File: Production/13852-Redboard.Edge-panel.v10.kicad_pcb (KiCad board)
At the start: 2 copper layers, 101.6 x 38.1 mm, 72 parts, among them J1 CONN_025MM, J17 QWIIC_CONNECTORJS-1MM, J2 CONN_03X2SMT, J20 POWER_JACKSMD, J4 USB_MICRO-B, J5 CONN_04, J6 CONN_04, Q1 MOSFET-SI2309DS, Q2 BSS138, Q3 BSS138, U1 CH340GSMD, U2 MIC5205-3.3V, U3 Standoff_Grounding, U4 ATMEGA328, U5 Standoff_Grounding, U6 LM1117, Y1 RESONATOR-16MHZ, Y2 CRYSTAL-12MHZ

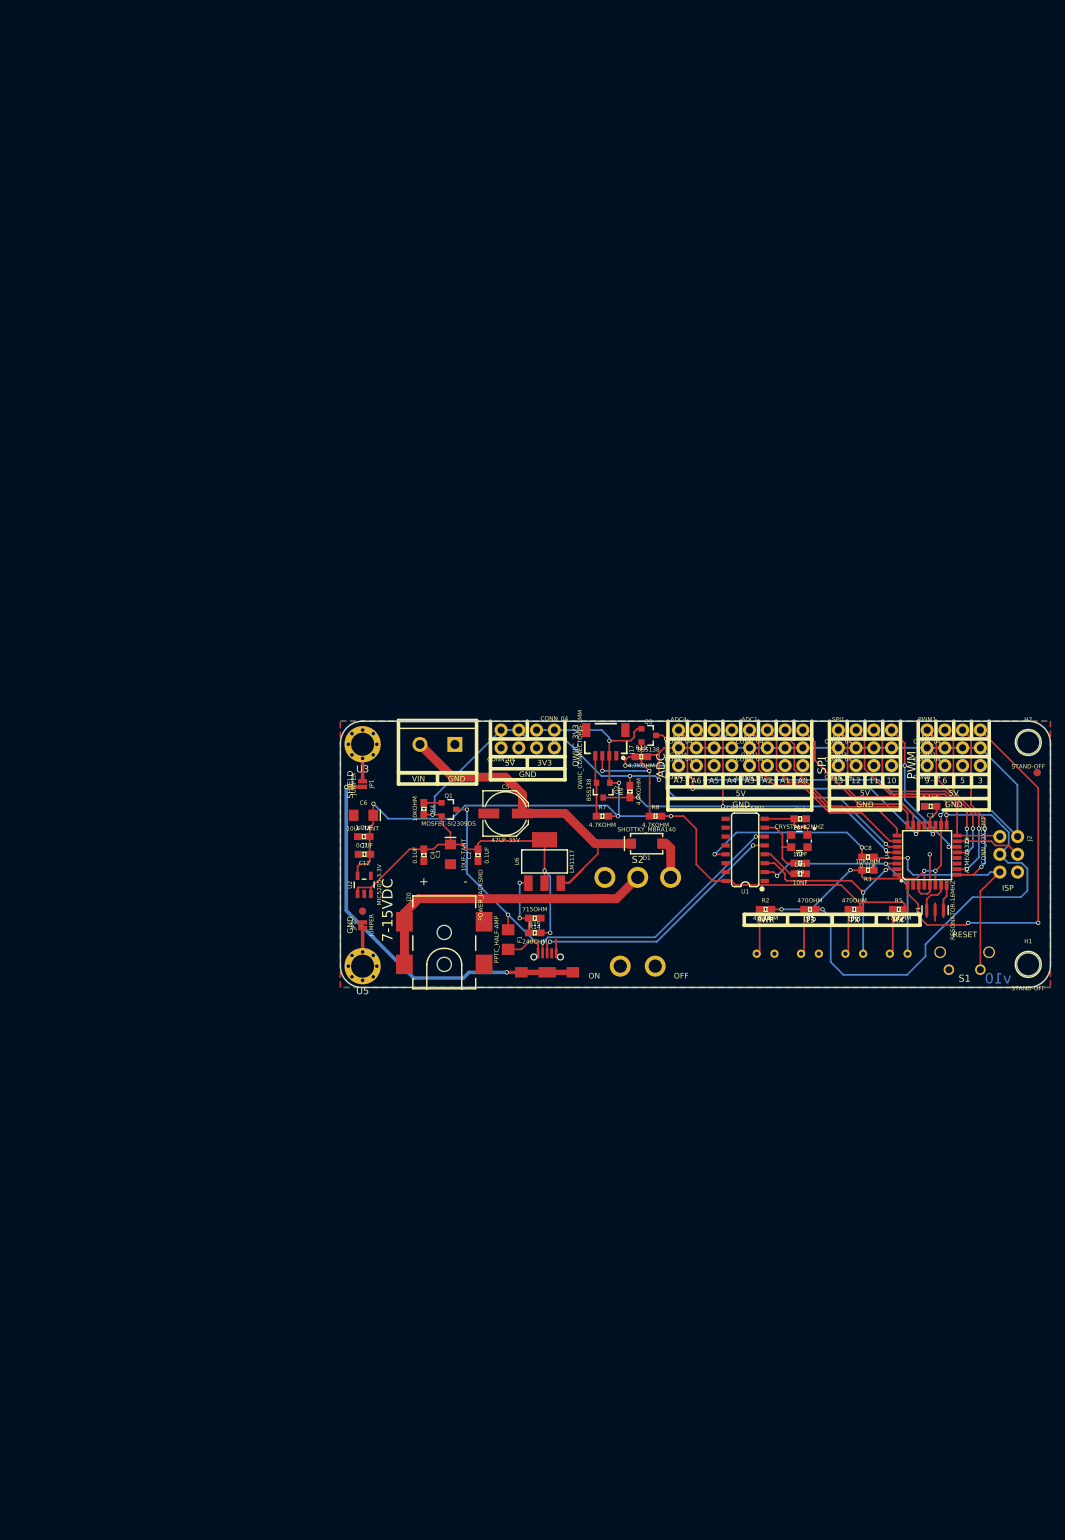
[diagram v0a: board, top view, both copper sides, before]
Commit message: panel
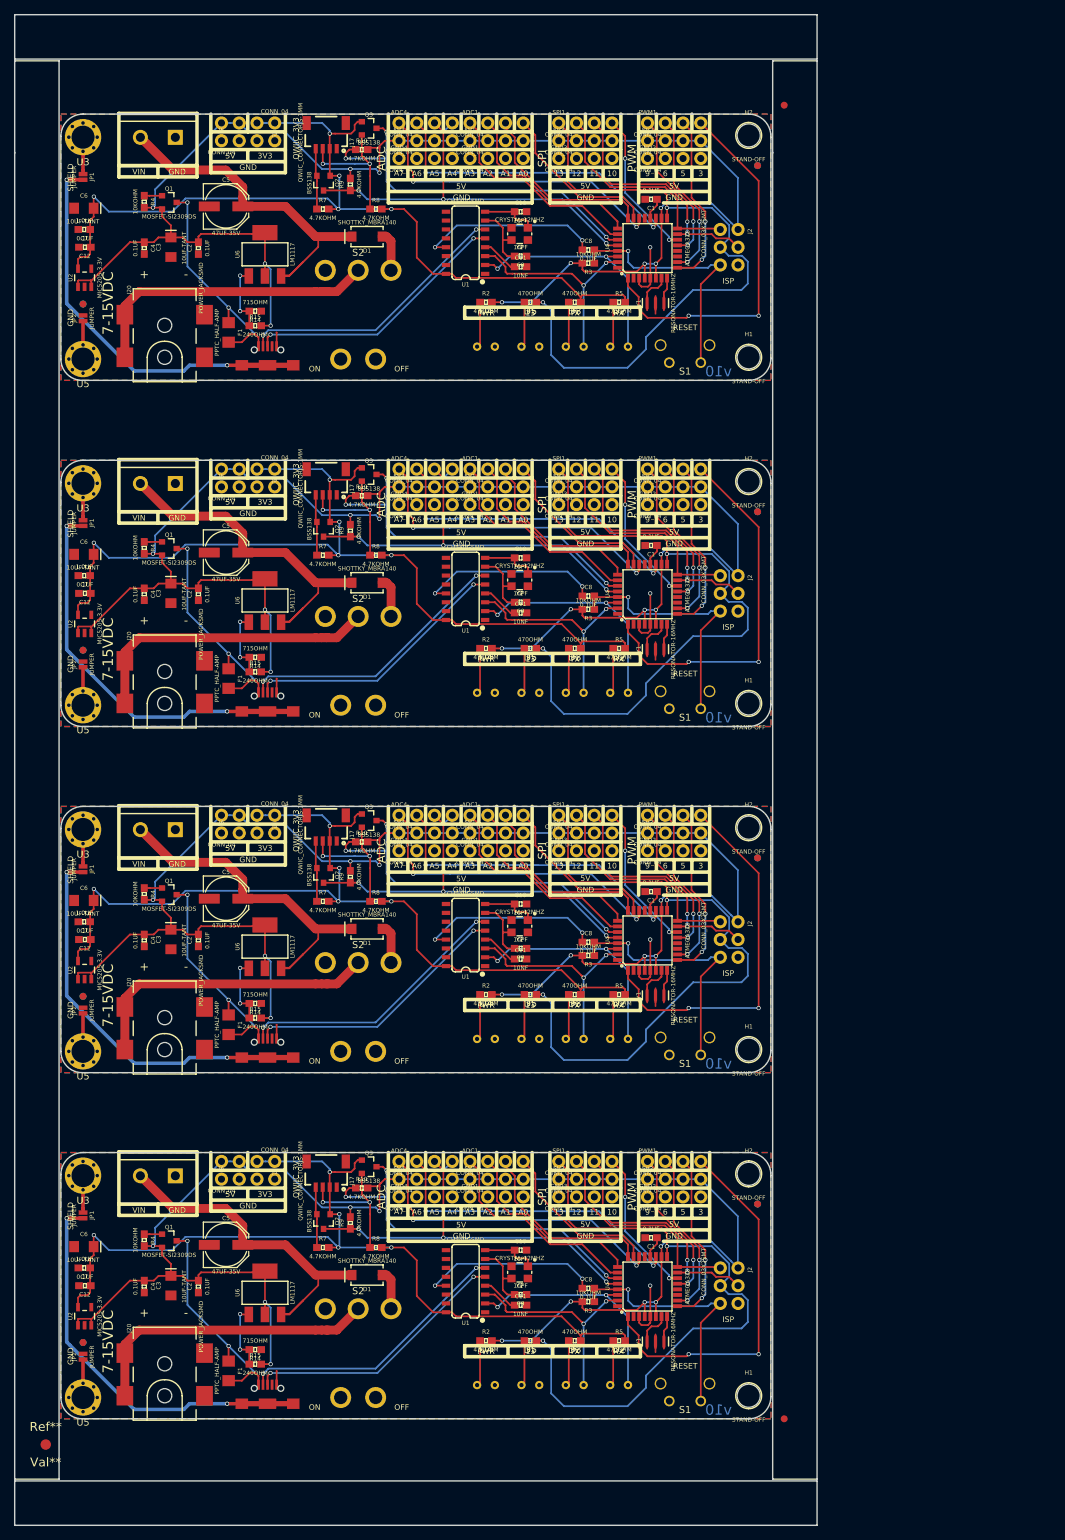
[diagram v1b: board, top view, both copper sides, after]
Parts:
- added 5V1: CONN_04, Connectors:1X04_NO_SILK, F.Cu at (119.5, -3.81)
- added 5V1: CONN_04, Connectors:1X04_NO_SILK, F.Cu at (119.5, 45.7)
- added 5V1: CONN_04, Connectors:1X04_NO_SILK, F.Cu at (119.5, 95.2)
- added 5V2: CONN_04, Connectors:1X04_NO_SILK, F.Cu at (144.9, -3.81)
- added 5V2: CONN_04, Connectors:1X04_NO_SILK, F.Cu at (144.9, 45.7)
- added 5V2: CONN_04, Connectors:1X04_NO_SILK, F.Cu at (144.9, 95.2)
- added 5V3: CONN_04, Connectors:1X04_NO_SILK, F.Cu at (132.2, -3.81)
- added 5V3: CONN_04, Connectors:1X04_NO_SILK, F.Cu at (132.2, 45.7)
- added 5V3: CONN_04, Connectors:1X04_NO_SILK, F.Cu at (132.2, 95.2)
- added 5V4: CONN_04, Connectors:1X04_NO_SILK, F.Cu at (109.3, -3.81)
- added 5V4: CONN_04, Connectors:1X04_NO_SILK, F.Cu at (109.3, 45.7)
- added 5V4: CONN_04, Connectors:1X04_NO_SILK, F.Cu at (109.3, 95.2)
- added ?: , Aesthetics:FIDUCIAL-1X2-no.paste, F.Cu at (164.5, 179.1)
- added ?: , Aesthetics:FIDUCIAL-1X2-no.paste, F.Cu at (164.5, -8.89)
- added ADC1: CONN_04, Connectors:1X04_NO_SILK, F.Cu at (119.5, -6.35)
- added ADC1: CONN_04, Connectors:1X04_NO_SILK, F.Cu at (119.5, 43.2)
- added ADC1: CONN_04, Connectors:1X04_NO_SILK, F.Cu at (119.5, 92.7)
- added ADC4: CONN_04, Connectors:1X04_NO_SILK, F.Cu at (109.3, -6.35)
- added ADC4: CONN_04, Connectors:1X04_NO_SILK, F.Cu at (109.3, 43.2)
- added ADC4: CONN_04, Connectors:1X04_NO_SILK, F.Cu at (109.3, 92.7)
- added C1: 0.1UF, Capacitors:0603, F.Cu at (145.4, 4.57)
- added C1: 0.1UF, Capacitors:0603, F.Cu at (145.4, 54.1)
- added C1: 0.1UF, Capacitors:0603, F.Cu at (145.4, 103.6)
- added C10: 10PF, Capacitors:0603, F.Cu at (126.7, 6.35)
- added C10: 10PF, Capacitors:0603, F.Cu at (126.7, 55.9)
- added C10: 10PF, Capacitors:0603, F.Cu at (126.7, 105.4)
- added C11: 10NF, Capacitors:0603, F.Cu at (126.7, 14.2)
- added C11: 10NF, Capacitors:0603, F.Cu at (126.7, 63.8)
- added C11: 10NF, Capacitors:0603, F.Cu at (126.7, 113.3)
- added C12: 0.1UF, Capacitors:0603, F.Cu at (64.4, 11.4)
- added C12: 0.1UF, Capacitors:0603, F.Cu at (64.4, 61.0)
- added C12: 0.1UF, Capacitors:0603, F.Cu at (64.4, 110.5)
- added C2: 0.1UF, Capacitors:0603, F.Cu at (80.6, 11.6)
- added C2: 0.1UF, Capacitors:0603, F.Cu at (80.6, 61.1)
- added C2: 0.1UF, Capacitors:0603, F.Cu at (80.6, 110.6)
- added C3: 10UF-TANT, Capacitors:EIA3216, F.Cu at (76.7, 11.4)
- added C3: 10UF-TANT, Capacitors:EIA3216, F.Cu at (76.7, 61.0)
- added C3: 10UF-TANT, Capacitors:EIA3216, F.Cu at (76.7, 110.5)
- added C4: 0.1UF, Capacitors:0603, F.Cu at (72.9, 11.6)
- added C4: 0.1UF, Capacitors:0603, F.Cu at (72.9, 61.1)
- added C4: 0.1UF, Capacitors:0603, F.Cu at (72.9, 110.6)
- added C5: 47UF-35V, Capacitors:PANASONIC_D, F.Cu at (84.6, 5.59)
- added C5: 47UF-35V, Capacitors:PANASONIC_D, F.Cu at (84.6, 55.1)
- added C5: 47UF-35V, Capacitors:PANASONIC_D, F.Cu at (84.6, 104.6)
- added C6: 10UF-TANT, Capacitors:EIA3216, F.Cu at (64.3, 5.84)
- added C6: 10UF-TANT, Capacitors:EIA3216, F.Cu at (64.3, 55.4)
- added C6: 10UF-TANT, Capacitors:EIA3216, F.Cu at (64.3, 104.9)
- added C7: 1.0UF, Capacitors:0603, F.Cu at (64.3, 8.89)
- added C7: 1.0UF, Capacitors:0603, F.Cu at (64.3, 58.4)
- added C7: 1.0UF, Capacitors:0603, F.Cu at (64.3, 108.0)
- added C8: 0.1UF, Capacitors:0603, F.Cu at (136.4, 11.8)
- added C8: 0.1UF, Capacitors:0603, F.Cu at (136.4, 61.3)
- added C8: 0.1UF, Capacitors:0603, F.Cu at (136.4, 110.9)
- added C9: 10PF, Capacitors:0603, F.Cu at (126.7, 12.7)
- added C9: 10PF, Capacitors:0603, F.Cu at (126.7, 62.2)
- added C9: 10PF, Capacitors:0603, F.Cu at (126.7, 111.8)
- added D1: SHOTTKY_MBRA140, Silicon-Standard:SMA-DIODE, F.Cu at (104.8, 9.91)
- added D1: SHOTTKY_MBRA140, Silicon-Standard:SMA-DIODE, F.Cu at (104.8, 59.4)
- added D1: SHOTTKY_MBRA140, Silicon-Standard:SMA-DIODE, F.Cu at (104.8, 109.0)
- added D2: LED-YELLOW, LED:LED_550_T1-.75_RT_ANG_PCB, F.Cu at (140.8, 25.7)
- added D2: LED-YELLOW, LED:LED_550_T1-.75_RT_ANG_PCB, F.Cu at (140.8, 75.2)
- added D2: LED-YELLOW, LED:LED_550_T1-.75_RT_ANG_PCB, F.Cu at (140.8, 124.7)
- added D3: LED-GREEN, LED:LED_550_T1-.75_RT_ANG_PCB, F.Cu at (134.5, 25.7)
- added D3: LED-GREEN, LED:LED_550_T1-.75_RT_ANG_PCB, F.Cu at (134.5, 75.2)
- added D3: LED-GREEN, LED:LED_550_T1-.75_RT_ANG_PCB, F.Cu at (134.5, 124.7)
- added D4: LED-RED, LED:LED_550_T1-.75_RT_ANG_PCB, F.Cu at (121.8, 25.7)
- added D4: LED-RED, LED:LED_550_T1-.75_RT_ANG_PCB, F.Cu at (121.8, 75.2)
- added D4: LED-RED, LED:LED_550_T1-.75_RT_ANG_PCB, F.Cu at (121.8, 124.7)
- added D5: LED-BLUE, LED:LED_550_T1-.75_RT_ANG_PCB, F.Cu at (128.1, 25.7)
- added D5: LED-BLUE, LED:LED_550_T1-.75_RT_ANG_PCB, F.Cu at (128.1, 75.2)
- added D5: LED-BLUE, LED:LED_550_T1-.75_RT_ANG_PCB, F.Cu at (128.1, 124.7)
- added F1: PPTC_HALF-AMP, Fuses:1206, F.Cu at (85.0, 23.6)
- added F1: PPTC_HALF-AMP, Fuses:1206, F.Cu at (85.0, 73.2)
- added F1: PPTC_HALF-AMP, Fuses:1206, F.Cu at (85.0, 122.7)
- added FD1: FIDUCIAL1X2, Aesthetics:FIDUCIAL-1X2, B.Cu at (160.7, -0.25)
- added FD1: FIDUCIAL1X2, Aesthetics:FIDUCIAL-1X2, B.Cu at (160.7, 49.3)
- added FD1: FIDUCIAL1X2, Aesthetics:FIDUCIAL-1X2, B.Cu at (160.7, 98.8)
- added FD2: FIDUCIAL1X2, Aesthetics:FIDUCIAL-1X2, F.Cu at (160.7, -0.25)
- added FD2: FIDUCIAL1X2, Aesthetics:FIDUCIAL-1X2, F.Cu at (160.7, 49.3)
- added FD2: FIDUCIAL1X2, Aesthetics:FIDUCIAL-1X2, F.Cu at (160.7, 98.8)
- added FD3: FIDUCIAL1X2, Aesthetics:FIDUCIAL-1X2, F.Cu at (64.1, 19.6)
- added FD3: FIDUCIAL1X2, Aesthetics:FIDUCIAL-1X2, F.Cu at (64.1, 69.1)
- added FD3: FIDUCIAL1X2, Aesthetics:FIDUCIAL-1X2, F.Cu at (64.1, 118.6)
- added FD4: FIDUCIAL1X2, Aesthetics:FIDUCIAL-1X2, B.Cu at (64.1, 19.6)
- added FD4: FIDUCIAL1X2, Aesthetics:FIDUCIAL-1X2, B.Cu at (64.1, 69.1)
- added FD4: FIDUCIAL1X2, Aesthetics:FIDUCIAL-1X2, B.Cu at (64.1, 118.6)
- added GND1: CONN_04, Connectors:1X04_NO_SILK, F.Cu at (119.5, -1.27)
- added GND1: CONN_04, Connectors:1X04_NO_SILK, F.Cu at (119.5, 48.3)
- added GND1: CONN_04, Connectors:1X04_NO_SILK, F.Cu at (119.5, 97.8)
- added GND2: CONN_04, Connectors:1X04_NO_SILK, F.Cu at (144.9, -1.27)
- added GND2: CONN_04, Connectors:1X04_NO_SILK, F.Cu at (144.9, 48.3)
- added GND2: CONN_04, Connectors:1X04_NO_SILK, F.Cu at (144.9, 97.8)
- added GND3: CONN_04, Connectors:1X04_NO_SILK, F.Cu at (132.2, -1.27)
- added GND3: CONN_04, Connectors:1X04_NO_SILK, F.Cu at (132.2, 48.3)
- added GND3: CONN_04, Connectors:1X04_NO_SILK, F.Cu at (132.2, 97.8)
- added GND4: CONN_04, Connectors:1X04_NO_SILK, F.Cu at (109.3, -1.27)
- added GND4: CONN_04, Connectors:1X04_NO_SILK, F.Cu at (109.3, 48.3)
- added GND4: CONN_04, Connectors:1X04_NO_SILK, F.Cu at (109.3, 97.8)
- added H1: STAND-OFF, Hardware:STAND-OFF, F.Cu at (159.4, 27.2)
- added H1: STAND-OFF, Hardware:STAND-OFF, F.Cu at (159.4, 76.7)
- added H1: STAND-OFF, Hardware:STAND-OFF, F.Cu at (159.4, 126.2)
- added H2: STAND-OFF, Hardware:STAND-OFF, F.Cu at (159.4, -4.57)
- added H2: STAND-OFF, Hardware:STAND-OFF, F.Cu at (159.4, 45.0)
- added H2: STAND-OFF, Hardware:STAND-OFF, F.Cu at (159.4, 94.5)
- added J1: CONN_025MM, Connectors:SCREWTERMINAL-5MM-2, F.Cu at (77.3, -4.29)
- added J1: CONN_025MM, Connectors:SCREWTERMINAL-5MM-2, F.Cu at (77.3, 45.2)
- added J1: CONN_025MM, Connectors:SCREWTERMINAL-5MM-2, F.Cu at (77.3, 94.8)
- added J17: QWIIC_CONNECTORJS-1MM, Connectors:1X04_1MM_RA, F.Cu at (98.9, -2.67)
- added J17: QWIIC_CONNECTORJS-1MM, Connectors:1X04_1MM_RA, F.Cu at (98.9, 46.9)
- added J17: QWIIC_CONNECTORJS-1MM, Connectors:1X04_1MM_RA, F.Cu at (98.9, 96.4)
- added J2: CONN_03X2SMT, Connectors:2X3-NS, F.Cu at (156.6, 11.4)
- added J2: CONN_03X2SMT, Connectors:2X3-NS, F.Cu at (156.6, 61.0)
- added J2: CONN_03X2SMT, Connectors:2X3-NS, F.Cu at (156.6, 110.5)
- added J20: POWER_JACKSMD, Connectors:POWER_JACK_SMD_GND, F.Cu at (75.8, 27.2)
- added J20: POWER_JACKSMD, Connectors:POWER_JACK_SMD_GND, F.Cu at (75.8, 76.7)
- added J20: POWER_JACKSMD, Connectors:POWER_JACK_SMD_GND, F.Cu at (75.8, 126.2)
- added J4: USB_MICRO-B, Connectors:USB-B-MICRO-SMD, F.Cu at (90.5, 28.3)
- added J4: USB_MICRO-B, Connectors:USB-B-MICRO-SMD, F.Cu at (90.5, 77.9)
- added J4: USB_MICRO-B, Connectors:USB-B-MICRO-SMD, F.Cu at (90.5, 127.4)
- added J5: CONN_04, Connectors:1X04_NO_SILK, F.Cu at (91.6, -6.35)
- added J5: CONN_04, Connectors:1X04_NO_SILK, F.Cu at (91.6, 43.2)
- added J5: CONN_04, Connectors:1X04_NO_SILK, F.Cu at (91.6, 92.7)
- added J6: CONN_04, Connectors:1X04_NO_SILK, F.Cu at (83.9, -3.81)
- added J6: CONN_04, Connectors:1X04_NO_SILK, F.Cu at (83.9, 45.7)
- added J6: CONN_04, Connectors:1X04_NO_SILK, F.Cu at (83.9, 95.2)
- added JP1: JUMPER, Jumpers:SMT-JUMPER_2_NO_NO-SILK, F.Cu at (64.1, 1.37)
- added JP1: JUMPER, Jumpers:SMT-JUMPER_2_NO_NO-SILK, F.Cu at (64.1, 50.9)
- added JP1: JUMPER, Jumpers:SMT-JUMPER_2_NO_NO-SILK, F.Cu at (64.1, 100.4)
- added JP2: JUMPER, Jumpers:SMT-JUMPER_2_NO_NO-SILK, F.Cu at (64.1, 21.6)
- added JP2: JUMPER, Jumpers:SMT-JUMPER_2_NO_NO-SILK, F.Cu at (64.1, 71.1)
- added JP2: JUMPER, Jumpers:SMT-JUMPER_2_NO_NO-SILK, F.Cu at (64.1, 120.7)
- added LOGO1: SFE_LOGO_NAME_FLAME.1_INCH, Aesthetics:SFE_LOGO_NAME_FLAME_.1, B.Cu at (83.4, 8.38)
- added LOGO1: SFE_LOGO_NAME_FLAME.1_INCH, Aesthetics:SFE_LOGO_NAME_FLAME_.1, B.Cu at (83.4, 57.9)
- added LOGO1: SFE_LOGO_NAME_FLAME.1_INCH, Aesthetics:SFE_LOGO_NAME_FLAME_.1, B.Cu at (83.4, 107.4)
- added LOGO2: OSHW-LOGOS, Aesthetics:OSHW-LOGO-S, B.Cu at (69.0, 6.35)
- added LOGO2: OSHW-LOGOS, Aesthetics:OSHW-LOGO-S, B.Cu at (69.0, 55.9)
- added LOGO2: OSHW-LOGOS, Aesthetics:OSHW-LOGO-S, B.Cu at (69.0, 105.4)
- added PWM1: CONN_04, Connectors:1X04_NO_SILK, F.Cu at (144.9, -6.35)
- added PWM1: CONN_04, Connectors:1X04_NO_SILK, F.Cu at (144.9, 43.2)
- added PWM1: CONN_04, Connectors:1X04_NO_SILK, F.Cu at (144.9, 92.7)
- added Q1: MOSFET-SI2309DS, Silicon-Standard:SOT23-3, F.Cu at (76.4, 5.01)
- added Q1: MOSFET-SI2309DS, Silicon-Standard:SOT23-3, F.Cu at (76.4, 54.5)
- added Q1: MOSFET-SI2309DS, Silicon-Standard:SOT23-3, F.Cu at (76.4, 104.1)
- added Q2: BSS138, Silicon-Standard:SOT23-3, F.Cu at (98.6, 2.20)
- added Q2: BSS138, Silicon-Standard:SOT23-3, F.Cu at (98.6, 51.7)
- added Q2: BSS138, Silicon-Standard:SOT23-3, F.Cu at (98.6, 101.3)
- added Q3: BSS138, Silicon-Standard:SOT23-3, F.Cu at (105.0, -5.59)
- added Q3: BSS138, Silicon-Standard:SOT23-3, F.Cu at (105.0, 43.9)
- added Q3: BSS138, Silicon-Standard:SOT23-3, F.Cu at (105.0, 93.5)
- added R1: 470OHM, Resistors:0603, F.Cu at (128.1, 19.3)
- added R1: 470OHM, Resistors:0603, F.Cu at (128.1, 68.8)
- added R1: 470OHM, Resistors:0603, F.Cu at (128.1, 118.4)
- added R10: 4.7KOHM, Resistors:0603, F.Cu at (104.0, -2.54)
- added R10: 4.7KOHM, Resistors:0603, F.Cu at (104.0, 47.0)
- added R10: 4.7KOHM, Resistors:0603, F.Cu at (104.0, 96.5)
- added R14: 715OHM, Resistors:0603, F.Cu at (88.8, 20.6)
- added R14: 715OHM, Resistors:0603, F.Cu at (88.8, 70.1)
- added R14: 715OHM, Resistors:0603, F.Cu at (88.8, 119.6)
- added R15: 240OHM, Resistors:0603, F.Cu at (88.8, 22.7)
- added R15: 240OHM, Resistors:0603, F.Cu at (88.8, 72.2)
- added R15: 240OHM, Resistors:0603, F.Cu at (88.8, 121.7)
- added R2: 470OHM, Resistors:0603, F.Cu at (121.8, 19.3)
- added R2: 470OHM, Resistors:0603, F.Cu at (121.8, 68.8)
- added R2: 470OHM, Resistors:0603, F.Cu at (121.8, 118.4)
- added R3: 10KOHM, Resistors:0603, F.Cu at (136.4, 13.7)
- added R3: 10KOHM, Resistors:0603, F.Cu at (136.4, 63.2)
- added R3: 10KOHM, Resistors:0603, F.Cu at (136.4, 112.8)
- added R4: 10KOHM, Resistors:0603, F.Cu at (72.9, 4.91)
- added R4: 10KOHM, Resistors:0603, F.Cu at (72.9, 54.4)
- added R4: 10KOHM, Resistors:0603, F.Cu at (72.9, 104.0)
- added R5: 470OHM, Resistors:0603, F.Cu at (140.8, 19.3)
- added R5: 470OHM, Resistors:0603, F.Cu at (140.8, 68.8)
- added R5: 470OHM, Resistors:0603, F.Cu at (140.8, 118.4)
- added R6: 470OHM, Resistors:0603, F.Cu at (134.5, 19.3)
- added R6: 470OHM, Resistors:0603, F.Cu at (134.5, 68.8)
- added R6: 470OHM, Resistors:0603, F.Cu at (134.5, 118.4)
- added R7: 4.7KOHM, Resistors:0603, F.Cu at (98.5, 5.97)
- added R7: 4.7KOHM, Resistors:0603, F.Cu at (98.5, 55.5)
- added R7: 4.7KOHM, Resistors:0603, F.Cu at (98.5, 105.0)
- added R8: 4.7KOHM, Resistors:0603, F.Cu at (106.0, 5.97)
- added R8: 4.7KOHM, Resistors:0603, F.Cu at (106.0, 55.5)
- added R8: 4.7KOHM, Resistors:0603, F.Cu at (106.0, 105.0)
- added R9: 4.7KOHM, Resistors:0603, F.Cu at (102.4, 2.45)
- added R9: 4.7KOHM, Resistors:0603, F.Cu at (102.4, 52.0)
- added R9: 4.7KOHM, Resistors:0603, F.Cu at (102.4, 101.5)
- added Ref**: Val**, Aesthetics:FIDUCIAL-FRAME-1_5MM-no.paste, F.Cu at (58.8, 182.8)
- added S1: MOMENTARY-SWITCH, Switches:SWITCH TACTILE SPST-NO 0.05A 12V, F.Cu at (150.3, 25.4)
- added S1: MOMENTARY-SWITCH, Switches:SWITCH TACTILE SPST-NO 0.05A 12V, F.Cu at (150.3, 75.0)
- added S1: MOMENTARY-SWITCH, Switches:SWITCH TACTILE SPST-NO 0.05A 12V, F.Cu at (150.3, 124.5)
- added S2: SWITCH_TOGGLE, Switches:TOGGLE_SWITCH-102-C3, F.Cu at (103.5, 13.5)
- added S2: SWITCH_TOGGLE, Switches:TOGGLE_SWITCH-102-C3, F.Cu at (103.5, 63.0)
- added S2: SWITCH_TOGGLE, Switches:TOGGLE_SWITCH-102-C3, F.Cu at (103.5, 112.5)
- added SPI1: CONN_04, Connectors:1X04_NO_SILK, F.Cu at (132.2, -6.35)
- added SPI1: CONN_04, Connectors:1X04_NO_SILK, F.Cu at (132.2, 43.2)
- added SPI1: CONN_04, Connectors:1X04_NO_SILK, F.Cu at (132.2, 92.7)
- added U1: CH340GSMD, Silicon-Standard:SO16, F.Cu at (118.9, 10.8)
- added U1: CH340GSMD, Silicon-Standard:SO16, F.Cu at (118.9, 60.3)
- added U1: CH340GSMD, Silicon-Standard:SO16, F.Cu at (118.9, 109.9)
- added U2: MIC5205-3.3V, Silicon-Standard:SOT23-5, F.Cu at (64.4, 15.8)
- added U2: MIC5205-3.3V, Silicon-Standard:SOT23-5, F.Cu at (64.4, 65.3)
- added U2: MIC5205-3.3V, Silicon-Standard:SOT23-5, F.Cu at (64.4, 114.9)
- added U3: Standoff_Grounding, Hardware:STANDOFF_GROUNDING, F.Cu at (64.1, -4.32)
- added U3: Standoff_Grounding, Hardware:STANDOFF_GROUNDING, F.Cu at (64.1, 45.2)
- added U3: Standoff_Grounding, Hardware:STANDOFF_GROUNDING, F.Cu at (64.1, 94.7)
- added U4: ATMEGA328, Silicon-Standard:TQFP32-08, F.Cu at (144.9, 11.6)
- added U4: ATMEGA328, Silicon-Standard:TQFP32-08, F.Cu at (144.9, 61.1)
- added U4: ATMEGA328, Silicon-Standard:TQFP32-08, F.Cu at (144.9, 110.6)
- added U5: Standoff_Grounding, Hardware:STANDOFF_GROUNDING, F.Cu at (64.1, 27.4)
- added U5: Standoff_Grounding, Hardware:STANDOFF_GROUNDING, F.Cu at (64.1, 77.0)
- added U5: Standoff_Grounding, Hardware:STANDOFF_GROUNDING, F.Cu at (64.1, 126.5)
- added U6: LM1117, Silicon-Standard:SOT223, F.Cu at (90.2, 12.4)
- added U6: LM1117, Silicon-Standard:SOT223, F.Cu at (90.2, 62.0)
- added U6: LM1117, Silicon-Standard:SOT223, F.Cu at (90.2, 111.5)
- added Y1: RESONATOR-16MHZ, Clocks:RESONATOR-SMD-3.2X1.3, F.Cu at (146.1, 19.4)
- added Y1: RESONATOR-16MHZ, Clocks:RESONATOR-SMD-3.2X1.3, F.Cu at (146.1, 69.0)
- added Y1: RESONATOR-16MHZ, Clocks:RESONATOR-SMD-3.2X1.3, F.Cu at (146.1, 118.5)
- added Y2: CRYSTAL-12MHZ, Clocks:CRYSTAL-SMD-3.2X2.5MM, F.Cu at (126.6, 9.53)
- added Y2: CRYSTAL-12MHZ, Clocks:CRYSTAL-SMD-3.2X2.5MM, F.Cu at (126.6, 59.1)
- added Y2: CRYSTAL-12MHZ, Clocks:CRYSTAL-SMD-3.2X2.5MM, F.Cu at (126.6, 108.6)
- moved R5 73.6 mm to (140.8, 167.9)
- moved 5V4 73.6 mm to (109.3, 144.8)
- moved ADC1 73.6 mm to (119.5, 142.2)
- moved ADC4 73.6 mm to (109.3, 142.2)
- moved C1 73.6 mm to (145.4, 153.2)
- moved C10 73.6 mm to (126.7, 154.9)
- moved C11 73.6 mm to (126.7, 162.8)
- moved C12 73.6 mm to (64.4, 160.0)
- moved C2 73.6 mm to (80.6, 160.1)
- moved C4 73.6 mm to (72.9, 160.1)
- moved C7 73.6 mm to (64.3, 157.5)
- moved C8 73.6 mm to (136.4, 160.4)
- moved C9 73.6 mm to (126.7, 161.3)
- moved D1 73.6 mm to (104.8, 158.5)
- moved D2 73.6 mm to (140.8, 174.2)
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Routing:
- net 5V: track 218.1 -> 872.5 mm, vias 10 -> 40
- net 3.3V: track 132.3 -> 529.2 mm, vias 5 -> 20
- net /SCK: track 92.7 -> 370.8 mm, vias 2 -> 8
- net VIN: track 63.7 -> 254.9 mm
- net /HI_SDA: track 63.4 -> 253.7 mm, vias 3 -> 12
- net /usb_shield: track 60.5 -> 241.9 mm, vias 2 -> 8
- net /HI_SCL: track 56.8 -> 227.1 mm, vias 3 -> 12
- net /PWM3: track 53.9 -> 215.5 mm, vias 2 -> 8
- net /AD7: track 45.3 -> 181.2 mm, vias 2 -> 8
- net /AD6: track 44.9 -> 179.7 mm, vias 2 -> 8
- net Net-(J20-PadVIN0): track 42.8 -> 171.4 mm
- net Net-(J4-PadD-): track 39.6 -> 158.4 mm, vias 2 -> 8
- net Net-(J4-PadD+): track 38.3 -> 153.0 mm, vias 2 -> 8
- net /RESET: track 37.2 -> 148.8 mm, vias 1 -> 4
- net /MOSI: track 35.4 -> 141.7 mm, vias 2 -> 8
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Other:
- board size 101.6 x 38.1 mm -> 114.8 x 216.2 mm
- board text added: "Route OUT"
- board text removed: "Designed by: Nick Poole"
- board text removed: "Standoff O.C."
